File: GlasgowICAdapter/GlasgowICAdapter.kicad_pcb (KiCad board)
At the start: 2 copper layers, 80 x 49 mm, 19 parts, among them J1 PORT A, J10 PORT A IO, J11 PORT B IO, J2 PORT B, J3 ZIF_SOCKET, J4 EN_U1, J5 EN_U2, J6 ZIF_IO_LEFT, J7 EN_U3, J8 EN_U4, J9 ZIF_IO_RIGHT, U1 TMUX1209RSVR, U2 TMUX1209RSVR, U4 TMUX1209RSVR, U5 TMUX1209RSVR

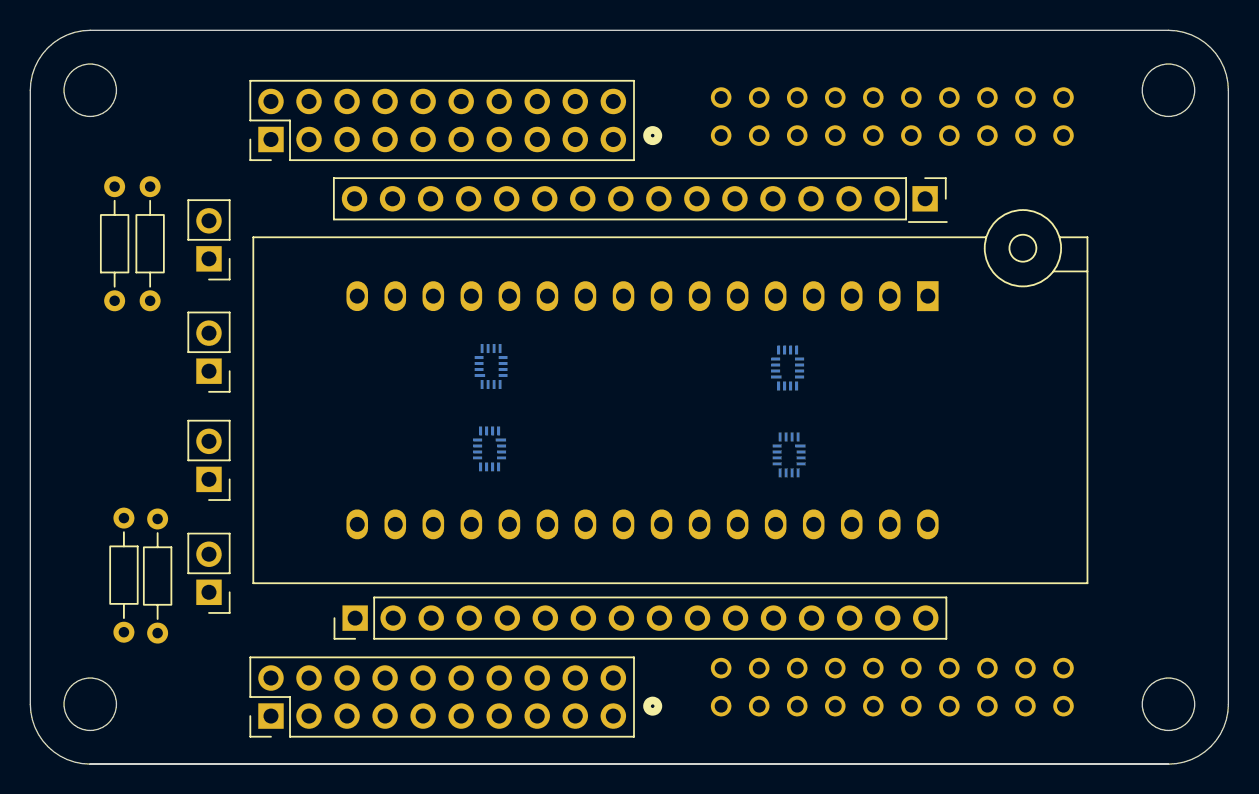
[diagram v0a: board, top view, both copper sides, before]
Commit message: Finished PCB routing, finally :D
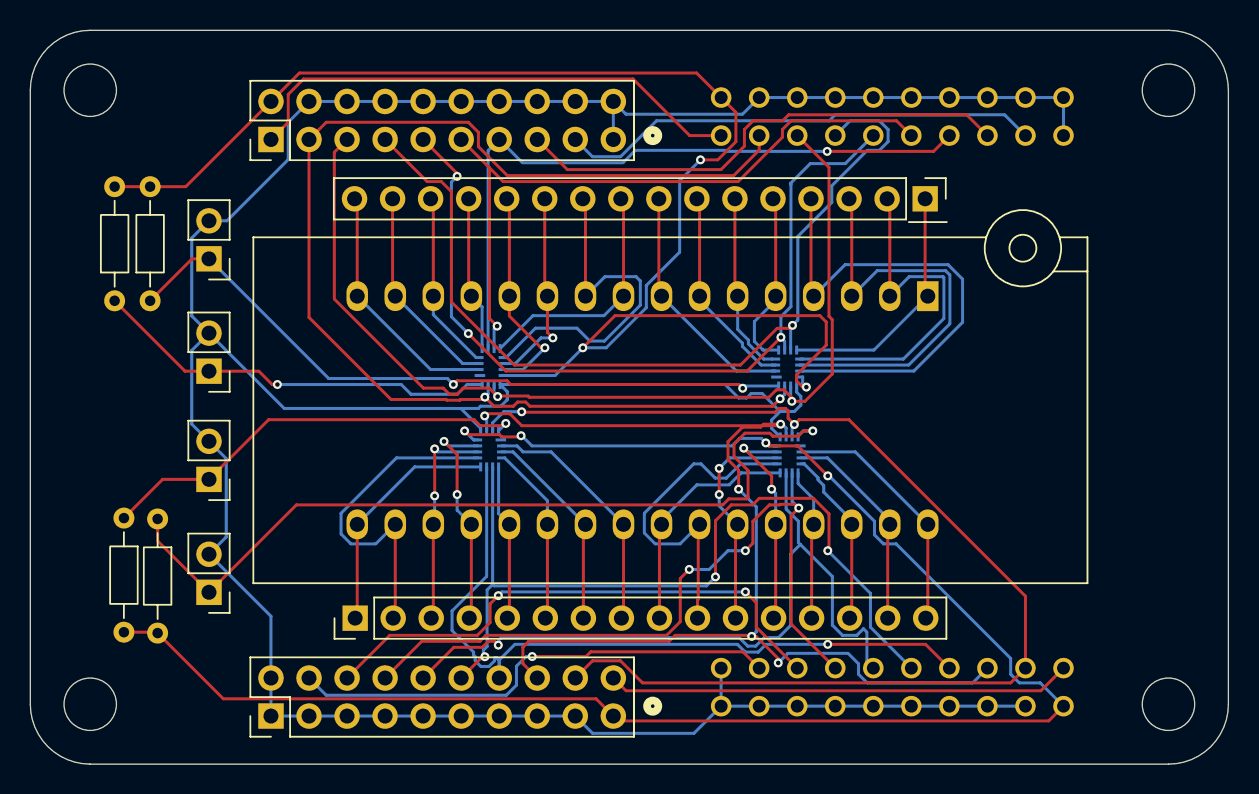
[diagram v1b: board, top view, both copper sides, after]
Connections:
- U1 pad 1: GND -> unconnected-(U1-NC-Pad1)
- U2 pad 1: GND -> unconnected-(U2-NC-Pad1)
- U4 pad 1: GND -> unconnected-(U4-NC-Pad1)
- U5 pad 1: GND -> unconnected-(U5-NC-Pad1)
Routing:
- net GND: track 0.00 -> 210.0 mm
- net VIOB: track 0.00 -> 116.8 mm, vias 0 -> 4
- net VIOA: track 0.00 -> 97.0 mm, vias 0 -> 3
- net PA0: track 0.00 -> 82.6 mm, vias 0 -> 2
- net PB0: track 0.00 -> 79.6 mm, vias 0 -> 2
- net PB1: track 0.00 -> 77.1 mm, vias 0 -> 5
- net PA1: track 0.00 -> 67.6 mm, vias 0 -> 2
- net PA2: track 0.00 -> 60.9 mm, vias 0 -> 1
- net Net-(J8-Pin_1): track 0.00 -> 55.8 mm, vias 0 -> 1
- net PA3: track 0.00 -> 55.7 mm, vias 0 -> 3
- net PB3: track 0.00 -> 55.4 mm, vias 0 -> 3
- net PB2: track 0.00 -> 50.7 mm, vias 0 -> 1
- net PB5: track 0.00 -> 49.7 mm, vias 0 -> 3
- net PB4: track 0.00 -> 49.4 mm, vias 0 -> 1
- net Net-(J4-Pin_1): track 0.00 -> 47.0 mm, vias 0 -> 2
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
